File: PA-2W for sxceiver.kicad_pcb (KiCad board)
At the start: 2 copper layers, 82.8 x 30.8 mm, 39 parts, among them J1 SMA_RF IN, J2 SMA_RF OUT, J3 5Vcc input, U1 TQP3M9036, U2 TQP7M9106

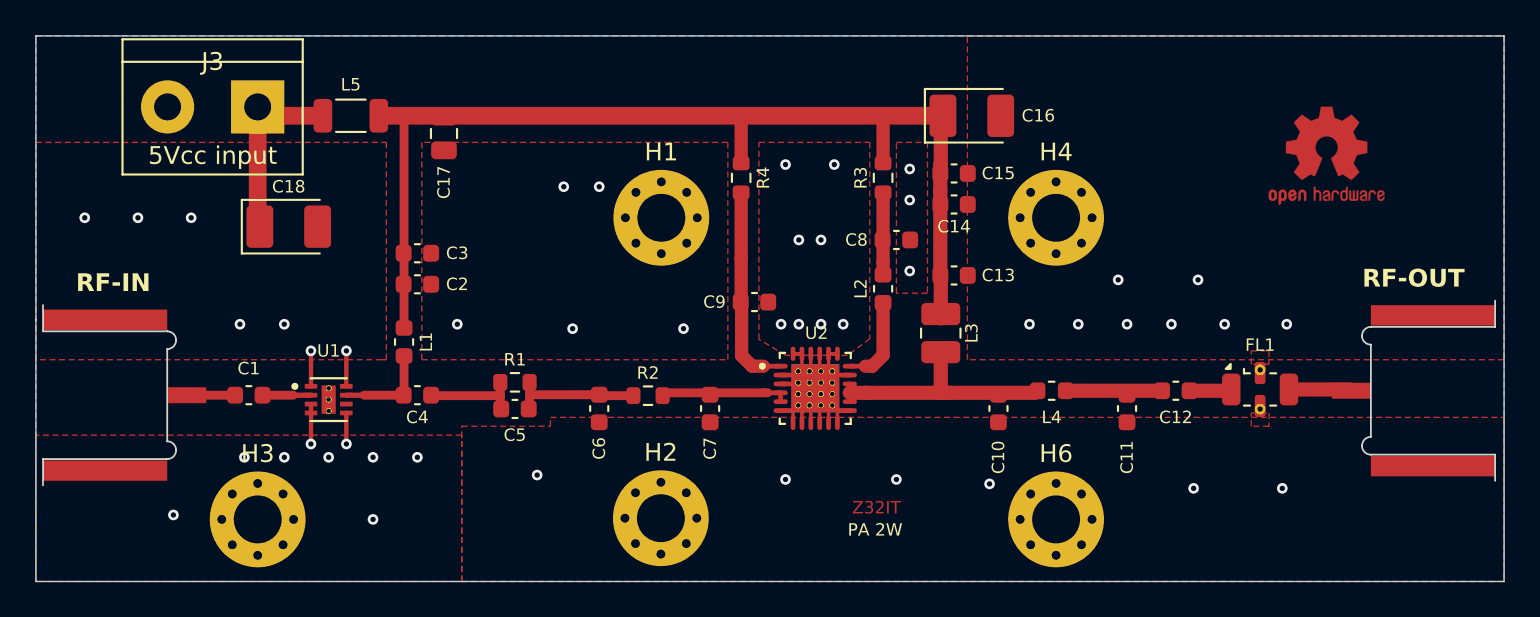
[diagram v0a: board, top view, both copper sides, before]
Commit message: Add files via upload
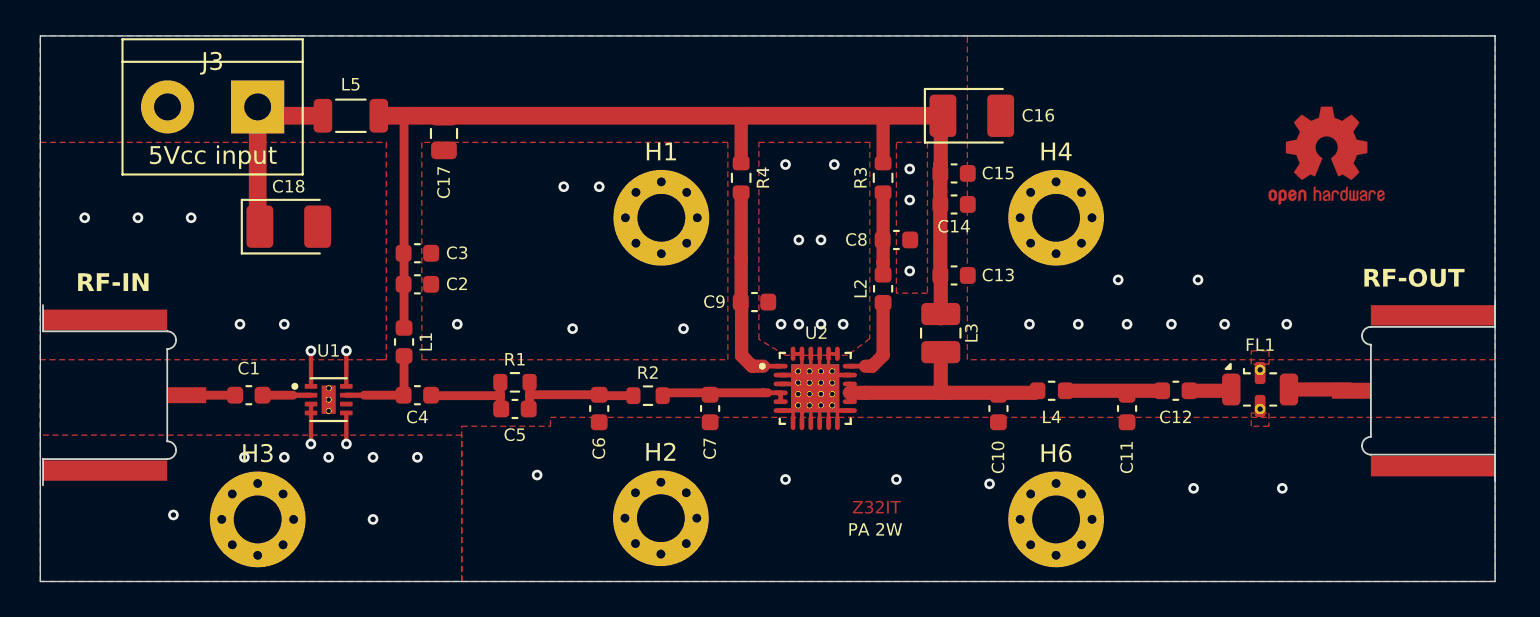
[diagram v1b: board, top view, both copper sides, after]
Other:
- board size 82.8 x 30.8 mm -> 82 x 30.8 mm
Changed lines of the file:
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@@
 	)
 	(gr_line
-		(start 91 88.75)
-		(end 173.75 88.75)
+		(start 91.25 88.75)
+		(end 173.24345 88.75)
 		(stroke
 			(width 0.05)
@@
 	)
 	(gr_line
-		(start 91 119.5)
-		(end 91 104.75)
+		(start 91.25 119.5)
+		(end 91.25 104.75)
 		(stroke
 			(width 0.05)
@@
 	)
 	(gr_line
-		(start 173.75 119.5)
-		(end 91 119.5)
+		(start 173.25 119.5)
+		(end 91.25 119.5)
 		(stroke
 			(width 0.05)
@@
 	)
 	(gr_line
-		(start 173.75 88.75)
-		(end 173.75 119.5)
+		(start 173.24345 88.75)
+		(end 173.24345 119.5)
 		(stroke
 			(width 0.05)
@@
 	)
 	(gr_line
-		(start 91 104.75)
-		(end 91 88.75)
+		(start 91.25 104.75)
+		(end 91.25 88.75)
 		(stroke
 			(width 0.05)
@@
 		(polygon
 			(pts
-				(xy 91 111.25) (xy 91 119.5) (xy 115 119.5) (xy 115 111.25)
+				(xy 91.25 111.25) (xy 91.25 119.5) (xy 115 119.5) (xy 115 111.25)
 			)
 		)
@@
 		(polygon
 			(pts
-				(xy 91 94.75) (xy 110.75 94.75) (xy 110.75 107) (xy 110.5 107) (xy 91 107)
+				(xy 91.25 94.75) (xy 110.75 94.75) (xy 110.75 107) (xy 110.5 107) (xy 91.25 107)
 			)
 		)
@@
 		(polygon
 			(pts
-				(xy 115 110.75) (xy 120 110.75) (xy 120 110.25) (xy 173.75 110.25) (xy 173.75 119.5) (xy 115 119.5)
+				(xy 115 110.75) (xy 120 110.75) (xy 120 110.25) (xy 173.25 110.25) (xy 173.25 119.5) (xy 115 119.5)
 			)
 		)
@@
 		(polygon
 			(pts
-				(xy 143.5 107) (xy 143.5 88.75) (xy 173.75 88.75) (xy 173.75 107)
+				(xy 143.5 107) (xy 143.5 88.75) (xy 173.25 88.75) (xy 173.25 107)
 			)
 		)
@@
 		(polygon
 			(pts
-				(xy 91 88.75) (xy 173.75 88.75) (xy 173.75 119.5) (xy 91 119.5)
+				(xy 91.25 88.75) (xy 173.25 88.75) (xy 173.25 119.5) (xy 91.25 119.5)
 			)
 		)
